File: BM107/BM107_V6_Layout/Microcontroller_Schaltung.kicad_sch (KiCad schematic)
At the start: 3 parts

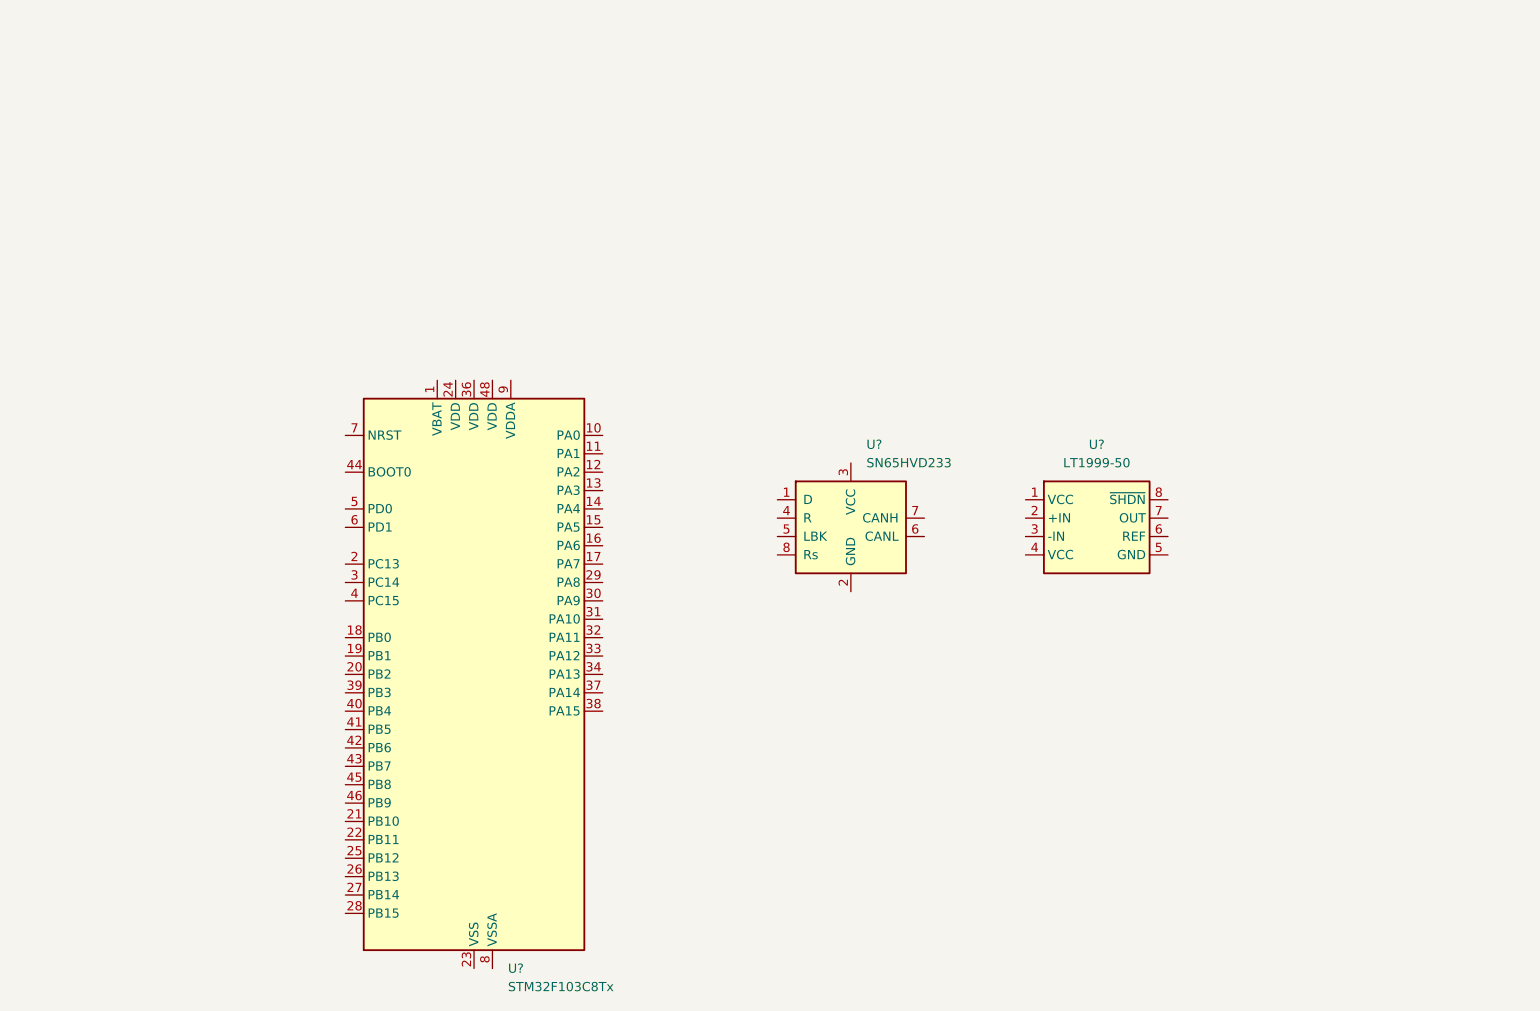
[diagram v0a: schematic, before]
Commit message: neuneuenu
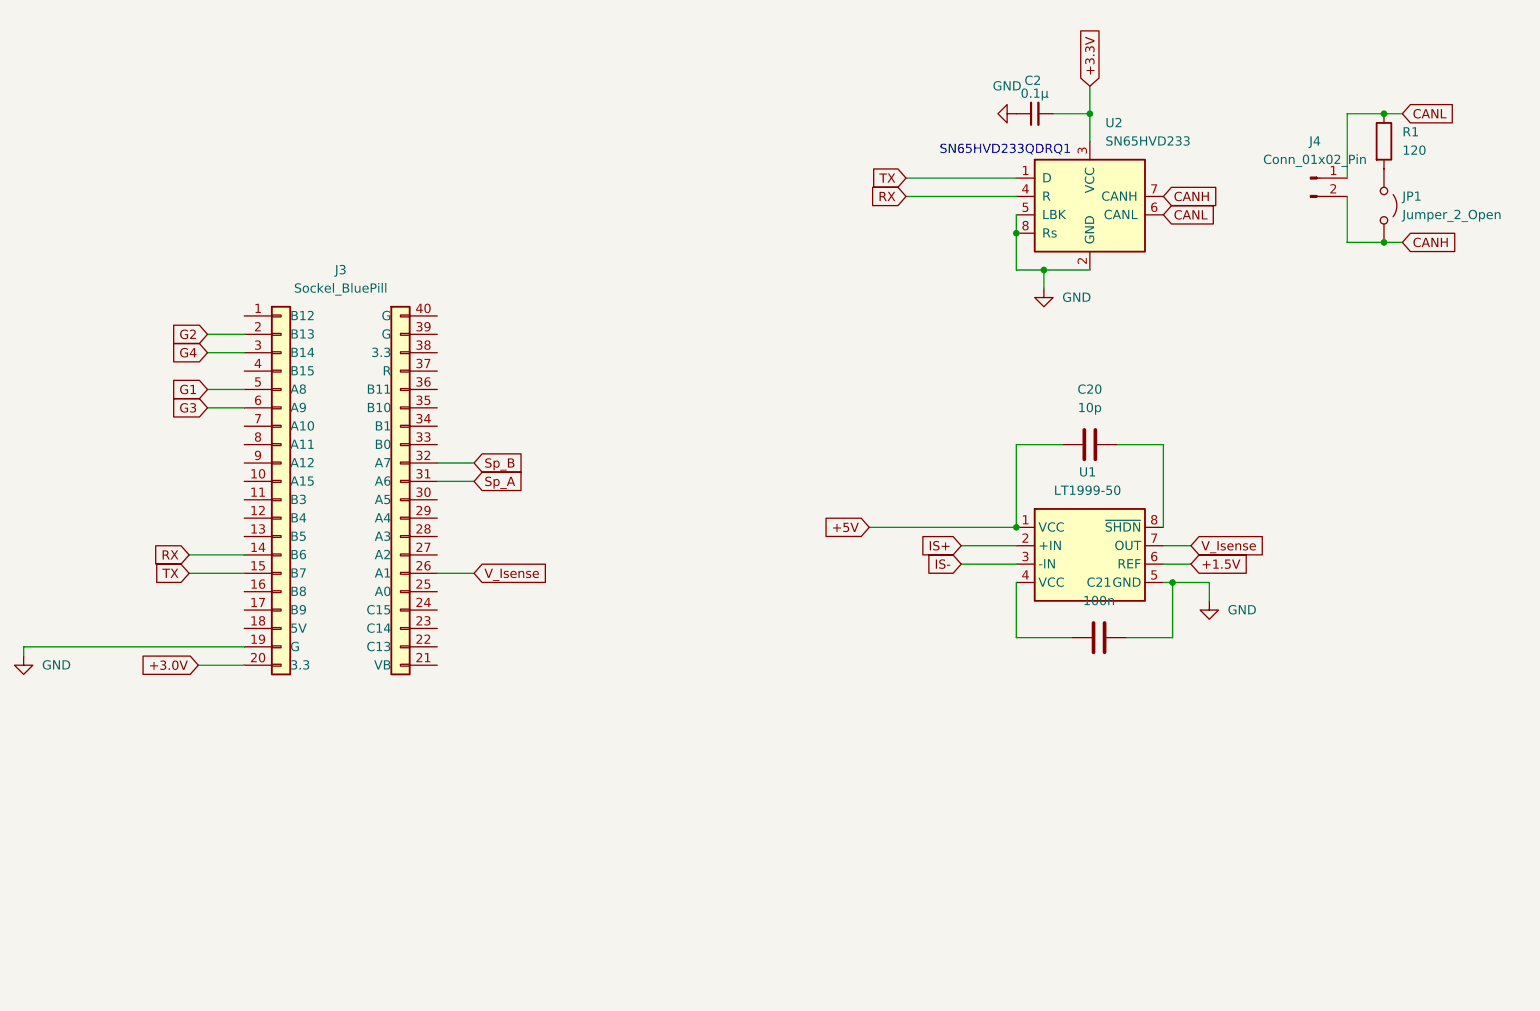
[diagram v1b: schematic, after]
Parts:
- removed U?: SN65HVD233, Package_SO:SOIC-8_3.9x4.9mm_P1.27mm, symbol Interface_CAN_LIN:SN65HVD233
- removed U?: STM32F103C8Tx, Package_QFP:LQFP-48_7x7mm_P0.5mm, symbol MCU_ST_STM32F1:STM32F103C8Tx
- removed U?: LT1999-50, Package_SO:MSOP-8_3x3mm_P0.65mm, symbol BM107_Labor_Lib:LT1999-50
- added C2: 0.1µ, Capacitor_SMD:C_0805_2012Metric, symbol Device:C_Small
- added C20: 10p, symbol Device:C
- added C21: 100n, symbol Device:C
- added J3: Sockel_BluePill, Aktive_Bal_Footprints:SockelBluepill Dupont leisten, symbol BM107:Sockel_BluePill
- added J4: Conn_01x02_Pin, Connector_PinHeader_2.54mm:PinHeader_1x02_P2.54mm_Vertical, symbol Connector:Conn_01x02_Pin
- added JP1: Jumper_2_Open, Jumper:SolderJumper-2_P1.3mm_Open_TrianglePad1.0x1.5mm, symbol Jumper:Jumper_2_Open
- added R1: 120, Resistor_SMD:R_0805_2012Metric, symbol Device:R
- added U1: LT1999-50, Package_SO:MSOP-8_3x3mm_P0.65mm, symbol BM107_Labor_Lib:LT1999-50
- added U2: SN65HVD233, Package_SO:SOIC-8_3.9x4.9mm_P1.27mm, symbol Interface_CAN_LIN:SN65HVD233
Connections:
- new net: C21.1, U1.4 (VCC)
- new net: C20.2, U1.8 (~{SHDN})
- new net: JP1.1 (A), R1.2
- new net +1.5V: U1.6 (REF)
- new net +3.0V: J3.20 (3.3)
- new net +3.3V: C2.2, U2.3 (VCC)
- new net +5V: C20.1, U1.1 (VCC)
- new net CANH: J4.2 (Pin_2), JP1.2 (B), U2.7 (CANH)
- new net CANL: J4.1 (Pin_1), R1.1, U2.6 (CANL)
- new net G1: J3.5 (A8)
- new net G2: J3.2 (B13)
- new net G3: J3.6 (A9)
- new net G4: J3.3 (B14)
- new net GND: C2.1, C21.2, J3.19 (G), U1.5 (GND), U2.2 (GND), U2.5 (LBK), U2.8 (Rs)
- new net IS+: U1.2 (+IN)
- new net IS-: U1.3 (-IN)
- new net RX: J3.14 (B6), U2.4 (R)
- new net Sp_A: J3.31 (A6)
- new net Sp_B: J3.32 (A7)
- new net TX: J3.15 (B7), U2.1 (D)
- new net V_Isense: J3.26 (A1), U1.7 (OUT)
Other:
- note added: "SN65HVD233QDRQ1"
